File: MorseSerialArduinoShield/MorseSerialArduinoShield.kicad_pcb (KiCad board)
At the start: 2 copper layers, 12 parts, among them U1 SC39-11SRWA

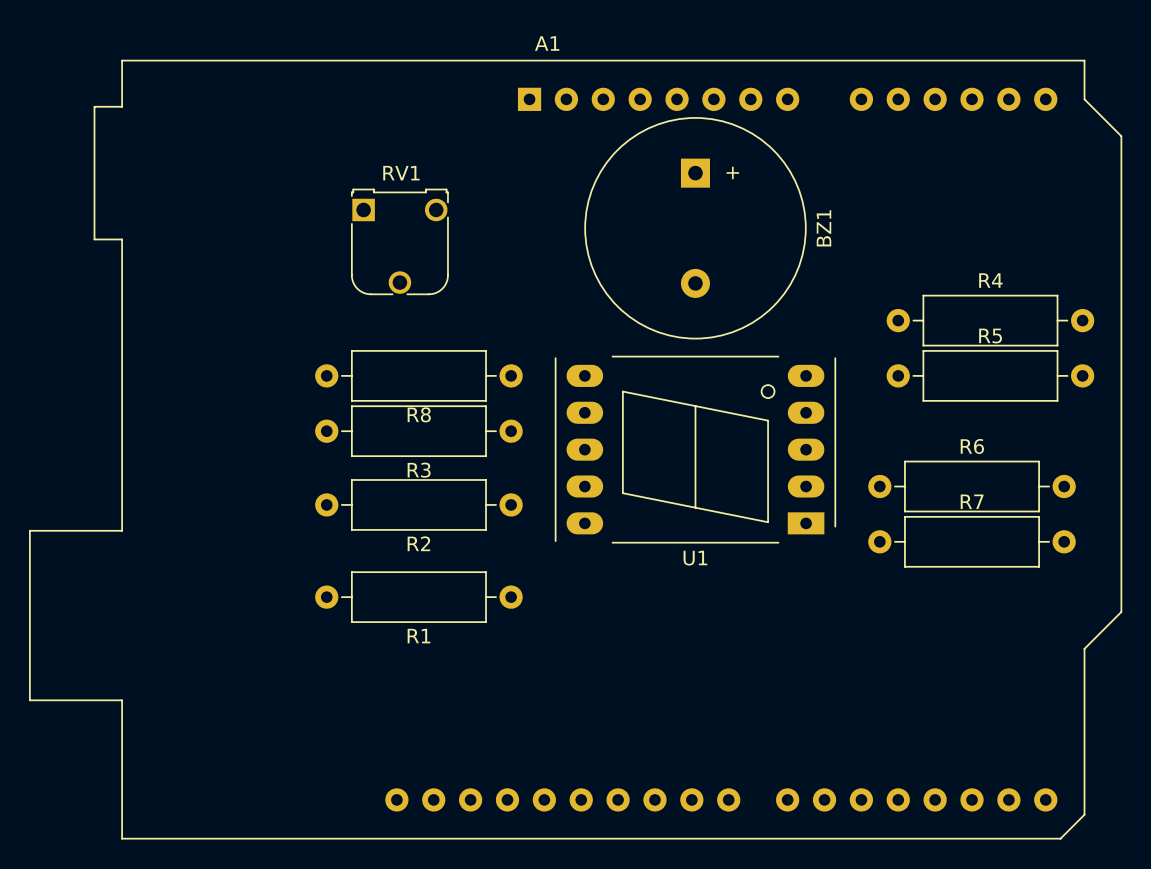
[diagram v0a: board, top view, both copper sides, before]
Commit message: startpoint
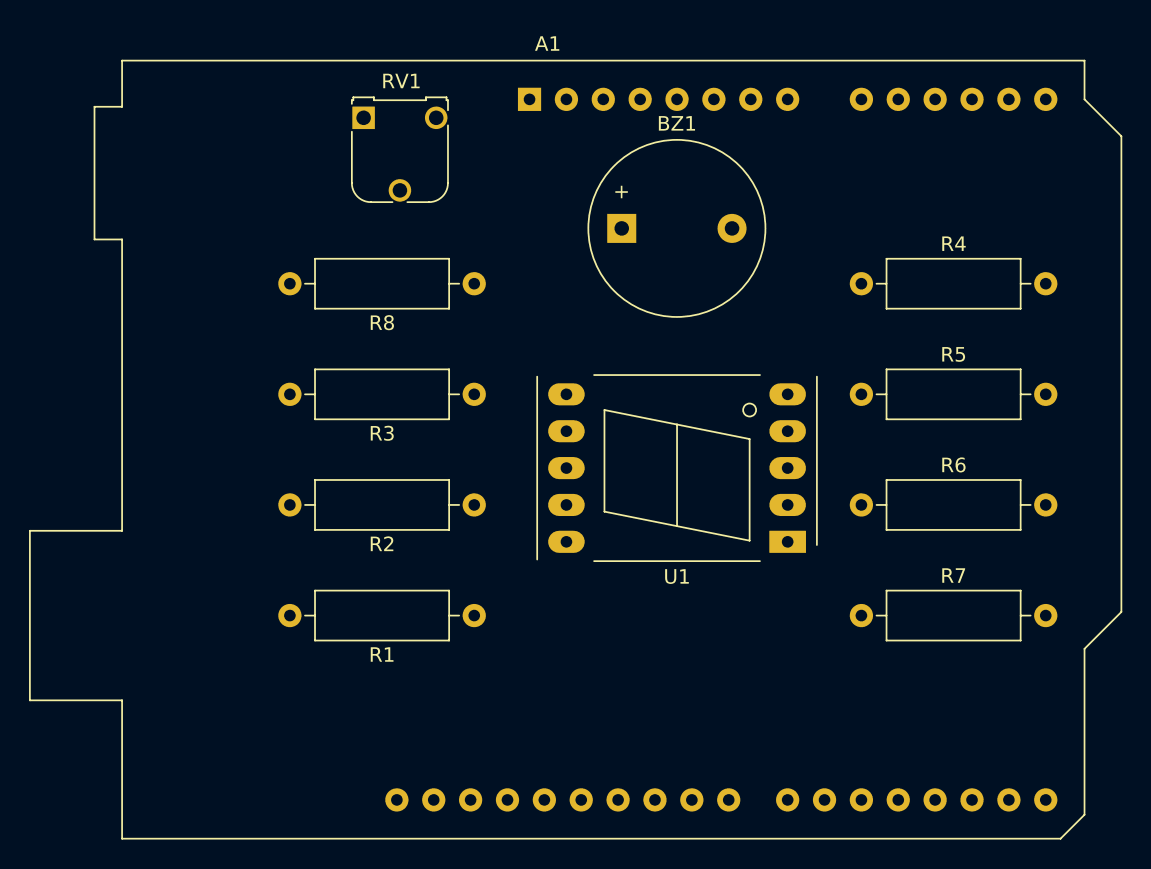
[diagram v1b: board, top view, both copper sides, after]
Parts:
- BZ1: footprint Buzzer_Beeper:Buzzer_15x7.5RM7.6 -> Buzzer_Beeper:Buzzer_12x9.5RM7.6
- moved R8 6.84 mm to (135.1, 88.3)
- moved RV1 6.35 mm to (127.5, 76.8)
- moved BZ1 6.35 mm to (145.3, 84.5), turned to 0 degrees
- moved R7 5.24 mm to (161.8, 111.1)
- moved R3 3.59 mm to (135.1, 95.9)
- moved R4 3.59 mm to (161.8, 88.3)
- moved R1 2.84 mm to (135.1, 111.1)
- moved R5 2.84 mm to (161.8, 95.9)
- moved R2 2.54 mm to (135.1, 103.5)
- moved R6 1.80 mm to (161.8, 103.5)
- moved U1 1.80 mm to (156.7, 106.0)
